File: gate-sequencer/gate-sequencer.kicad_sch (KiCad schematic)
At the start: 153 parts, among them J1 Power, J10 Gate 6, J11 Gate 7, J12 Gate 8, J13 Gate 9, J14 Gate 10, J15 Gate 11, J16 Gate 13, J17 Gate 12, J18 Gate 14, J19 Gate 15, J2 Power, J20 Gate 16, J21 Conn_01x34_Socket, J22 Clock, J23 Gate 1, J24 LED, J25 Gate 2, J26 LED, J27 LED, J28 LED, J29 Gate 3, J3 Power, J30 Gate 4, J31 Gate 5, J32 LED, J33 LED, J34 Gate 6, J35 LED, J36 LED, J37 Gate 7, J38 Gate 8, J39 LED, J4 Clock, J40 Gate 9, J41 LED, J42 Gate 10, J43 LED, J44 Gate 11, J45 LED, J46 LED, J47 Gate 13, J48 Gate 12, J49 Gate 14, J5 Gate 1, J50 LED, J51 Gate 15, J52 LED, J53 LED, J54 Gate 16, J55 Conn_01x34_Pin, J6 Gate 2, J7 Gate 3, J8 Gate 5, J9 Gate 4, SW1 Mode 2, SW10 S3, SW11 S4, SW12 S5, SW13 S6, SW14 S7, SW15 S8, SW16 S9, SW17 S10, SW18 S11, SW19 S12, SW2 Mode, SW20 S13, SW21 S14, SW22 S15, SW23 S16, SW3 Clock Source, SW4 X1, SW5 X2, SW6 X3, SW7 X4, SW8 S1, SW9 S2

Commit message: Update some designs
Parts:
- U1: value ~ -> (none)

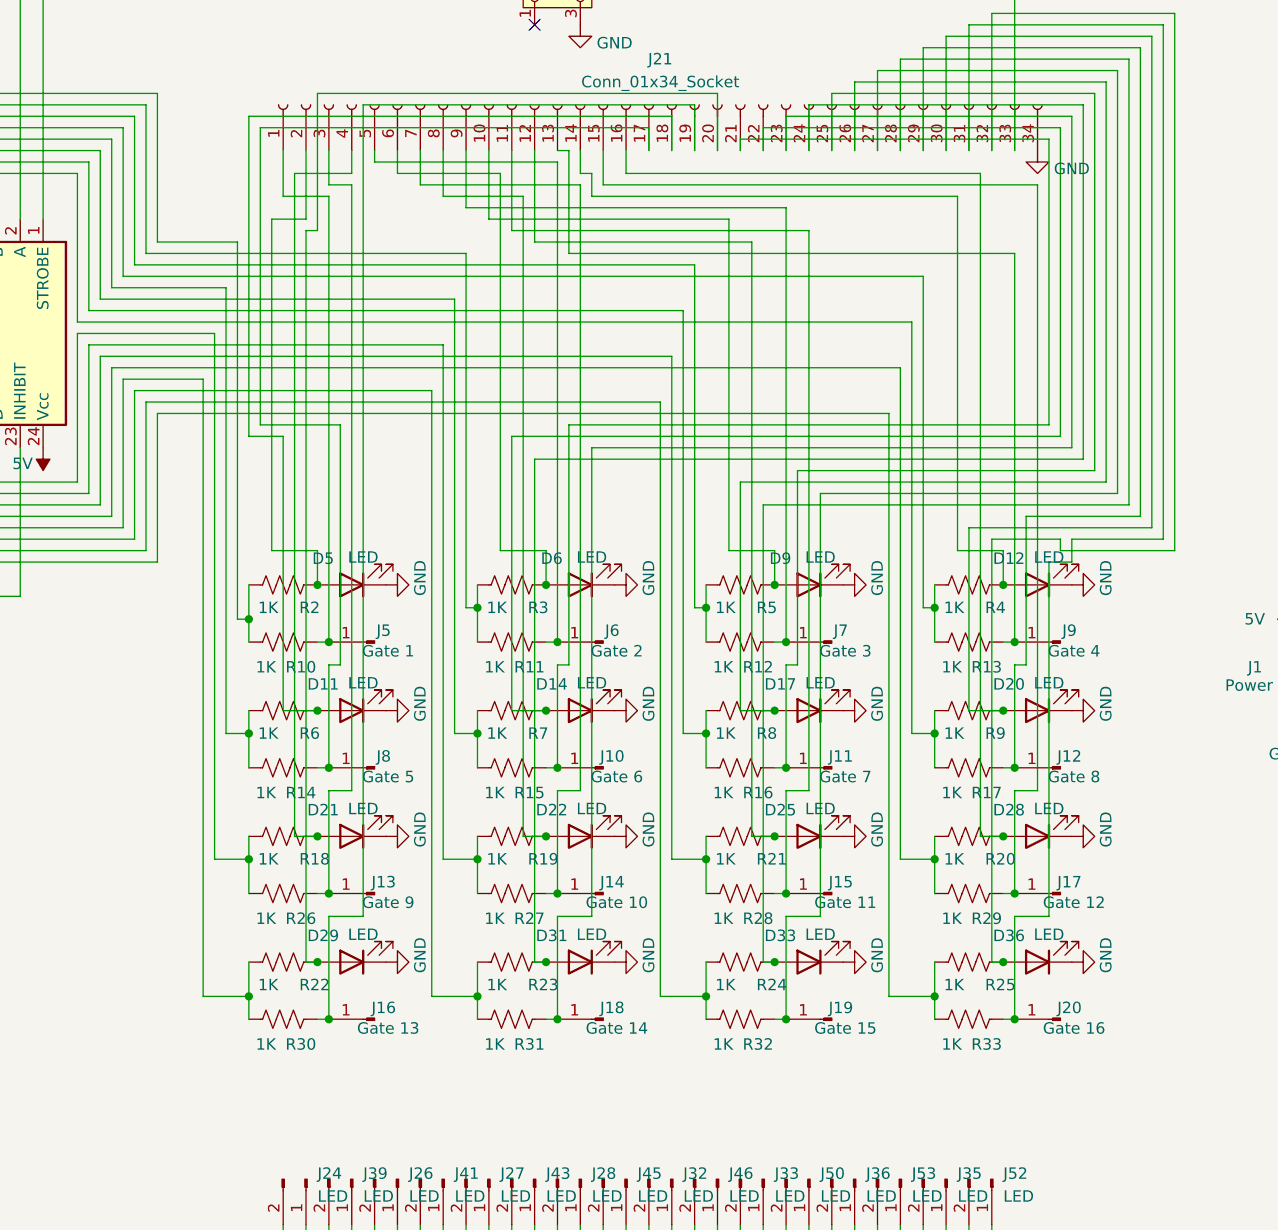
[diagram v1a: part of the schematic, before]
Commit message: Gate sequencer fixes
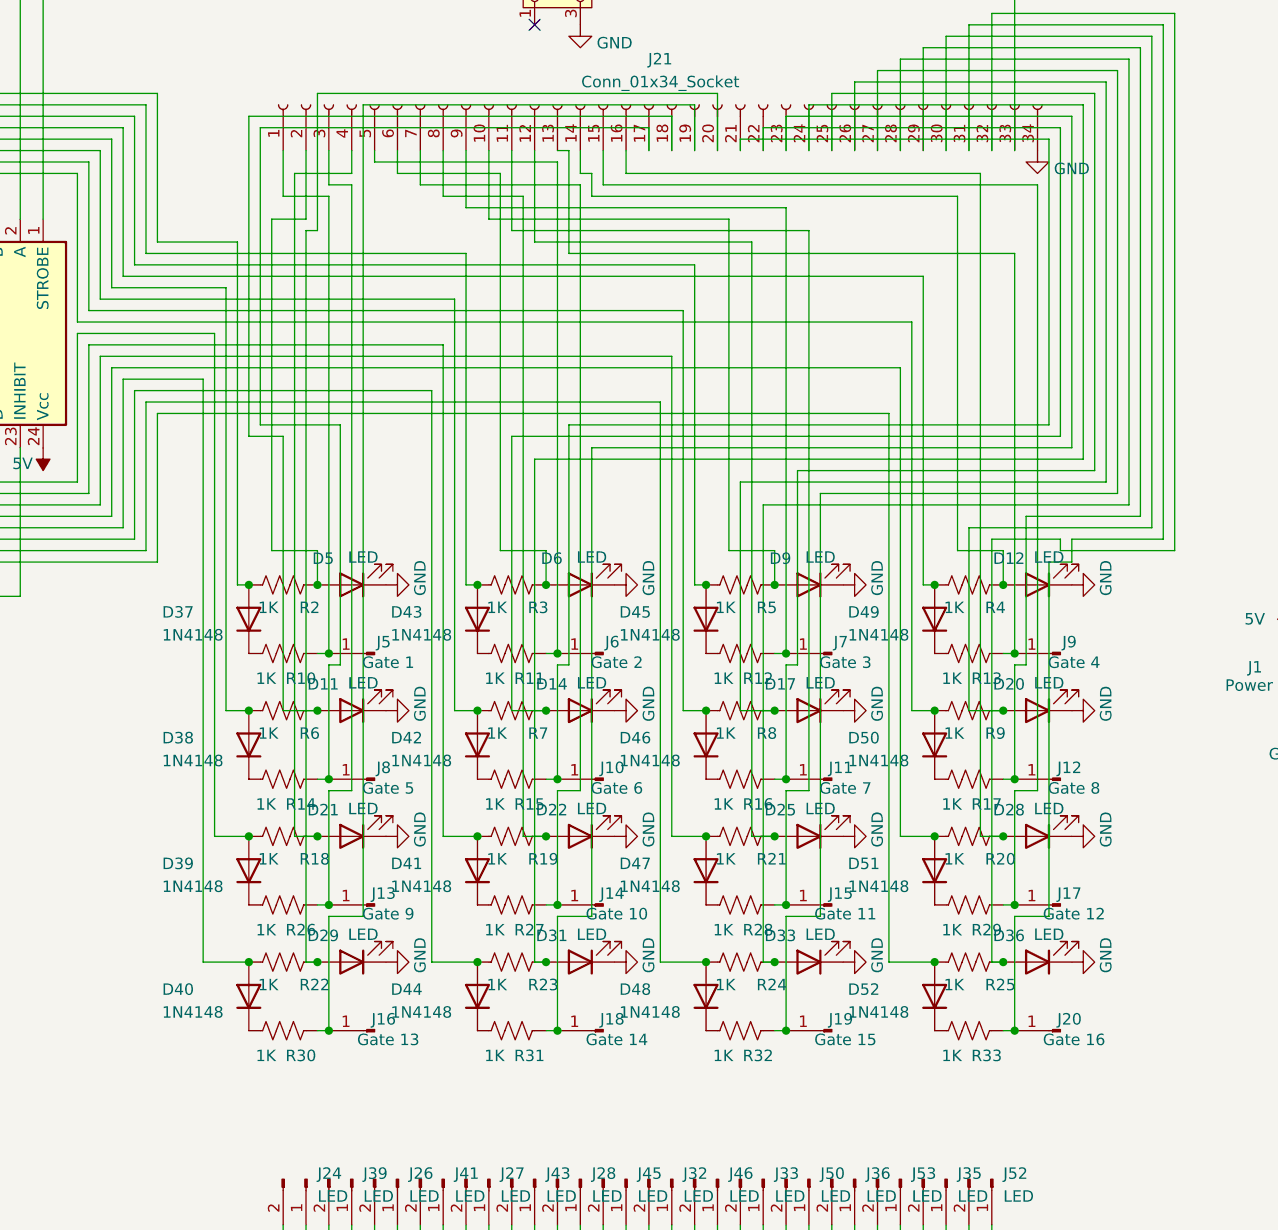
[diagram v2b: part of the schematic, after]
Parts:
- added D37, D38, D39, D40, D41, D42, D43, D44, D45, D46, D47, D48, D49, D50, D51, D52: 1N4148, Diode_THT:D_DO-35_SOD27_P7.62mm_Horizontal, symbol Diode:1N4148
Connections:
- net at R5.2, U1.10 (S2): now also D45.2 (A); no longer R12.2
- net at R20.2, U1.19 (S11): now also D51.2 (A); no longer R29.2
- net at R24.2, U1.16 (S14): now also D48.2 (A); no longer R32.2
- net at R9.2, U1.4 (S7): now also D50.2 (A); no longer R17.2
- net at R25.2, U1.15 (S15): now also D52.2 (A); no longer R33.2
- net at R23.2, U1.13 (S13): now also D44.2 (A); no longer R31.2
- net at R19.2, U1.17 (S9): now also D41.2 (A); no longer R27.2
- net at R18.2, U1.18 (S8): now also D39.2 (A); no longer R26.2
- net at R7.2, U1.6 (S5): now also D42.2 (A); no longer R15.2
- net at R8.2, U1.5 (S6): now also D46.2 (A); no longer R16.2
- net at R2.2, U1.11 (S0): now also D37.2 (A); no longer R10.2
- net at R22.2, U1.14 (S12): now also D40.2 (A); no longer R30.2
- net at R21.2, U1.20 (S10): now also D47.2 (A); no longer R28.2
- net at R6.2, U1.7 (S4): now also D38.2 (A); no longer R14.2
- net at R4.2, U1.8 (S3): now also D49.2 (A); no longer R13.2
- net at R3.2, U1.9 (S1): now also D43.2 (A); no longer R11.2
- new net: D41.1 (K), R27.2
- new net: D45.1 (K), R12.2
- new net: D50.1 (K), R17.2
- new net: D48.1 (K), R32.2
- new net: D40.1 (K), R30.2
- new net: D49.1 (K), R13.2
- new net: D52.1 (K), R33.2
- new net: D39.1 (K), R26.2
- new net: D38.1 (K), R14.2
- new net: D42.1 (K), R15.2
- new net: D46.1 (K), R16.2
- new net: D44.1 (K), R31.2
- new net: D51.1 (K), R29.2
- new net: D43.1 (K), R11.2
- new net: D47.1 (K), R28.2
- new net: D37.1 (K), R10.2
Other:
- moved on the sheet: J10, J11, J12, J13, J14, J15, J16, J17, J18, J19, J20, J5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
